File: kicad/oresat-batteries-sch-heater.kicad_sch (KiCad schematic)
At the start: 20 parts, among them Q20 PMV45ENR, Q21 PMV45ENR, Q38 PMV45ENR, Q39 PMV45ENR, Q42 DMP2240UDM-7, Q43 DMP2240UDM-7

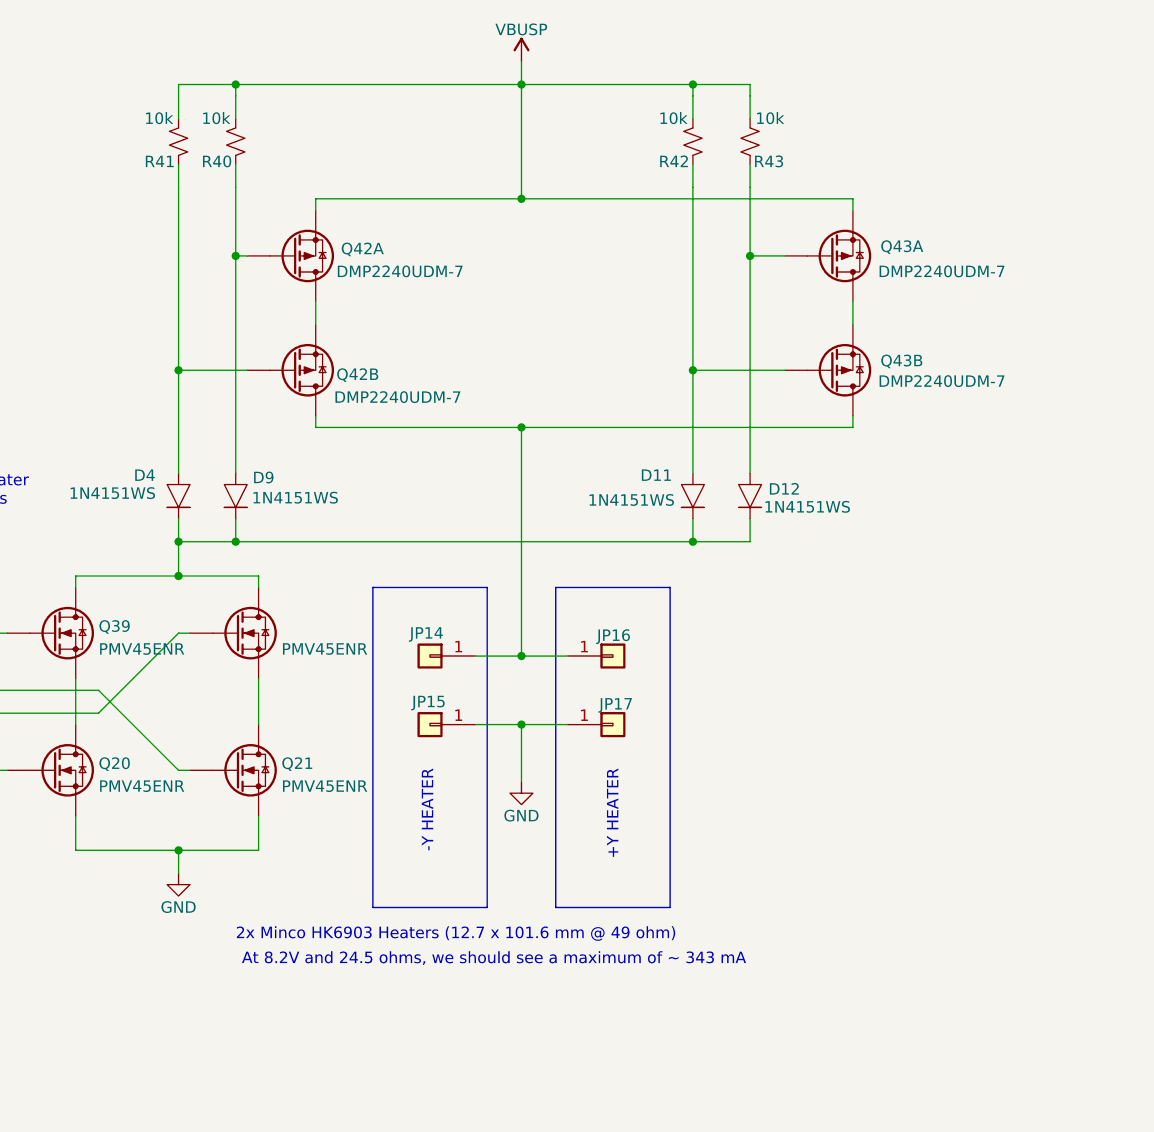
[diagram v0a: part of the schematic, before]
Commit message: Not sure what changed from back in February, but committing anyway :)
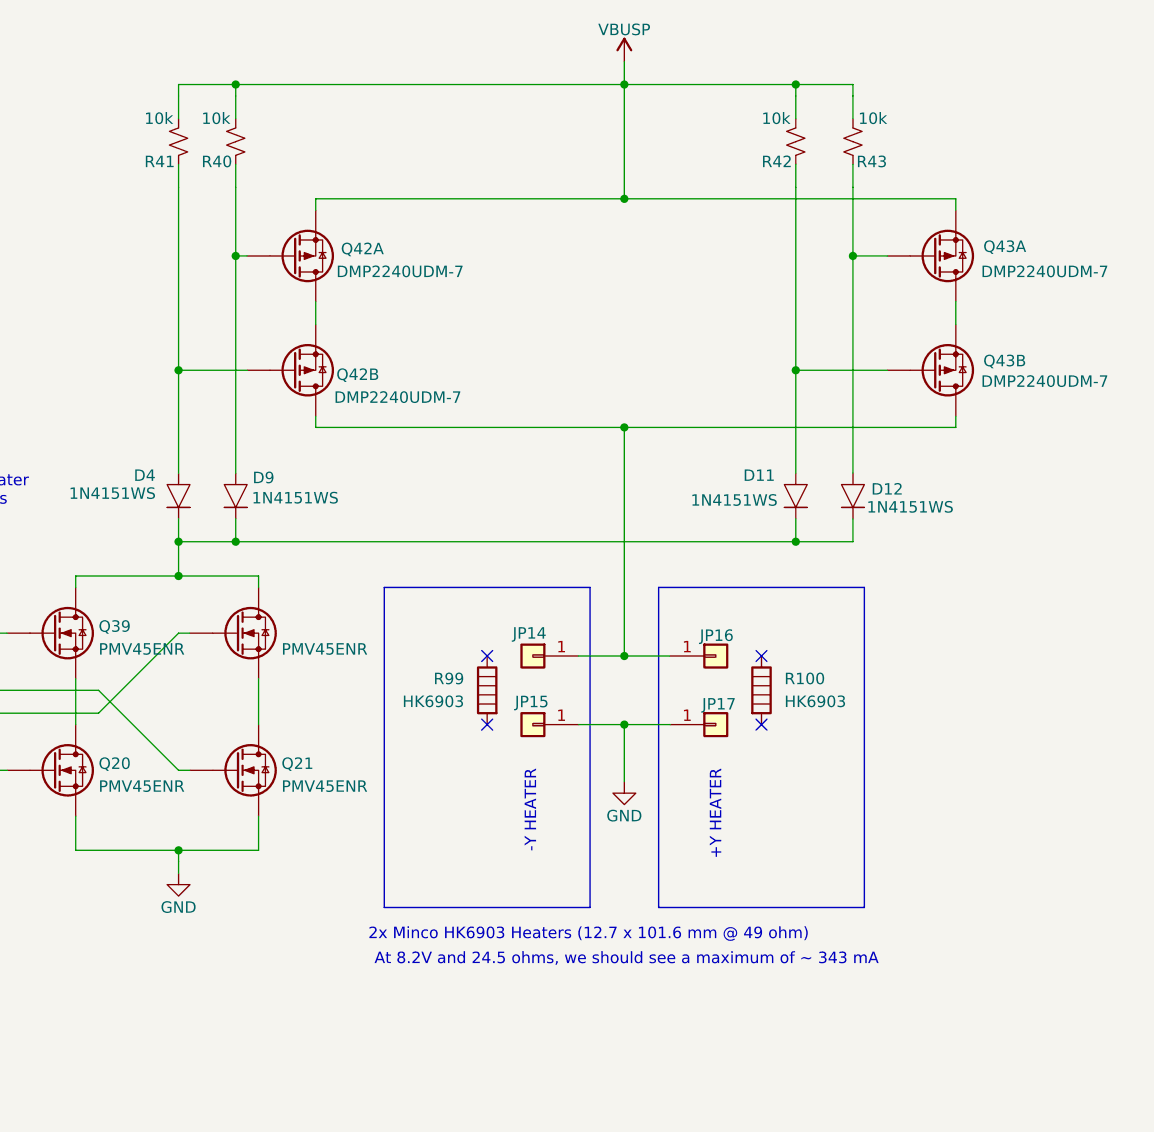
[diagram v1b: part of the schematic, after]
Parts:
- added R100, R99: HK6903, symbol Device:Heater
- D11, D12, D4, D9: DIS (none) -> DigiKey; DPN (none) -> 112-1N4151WS-E3-08CT-ND; MFR (none) -> Vishay; MPN (none) -> 1N4151WS-E3-08
- JP14, JP15, JP16, JP17: DIS (none) -> N/A; DPN (none) -> N/A; MFR (none) -> N/A; MPN (none) -> N/A; now left out of the parts list
- R105, R106, R40, R41, R42, R43: DIS Digi-Key -> DigiKey; DPN 311-10.0KHRCT-ND -> RMCF0603FT10K0CT-ND; MFR Yageo -> Stackpole Electronics; MPN RC0603FR-0710KL -> RMCF0603FT10K0
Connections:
- no-connect marks 0 -> 4
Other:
- moved on the sheet: D11, D12, JP14, JP15, JP16, JP17, Q43A, Q43B, R42, R43
